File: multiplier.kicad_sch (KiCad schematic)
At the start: 4 parts, among them U12 4081, U2 4081, U37 4069, U7 4081

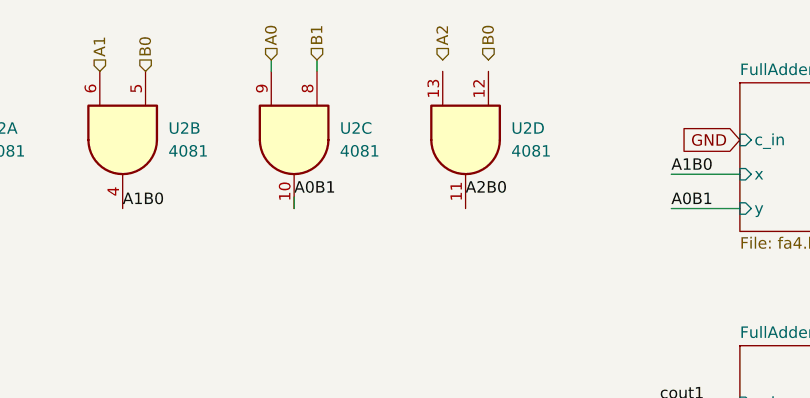
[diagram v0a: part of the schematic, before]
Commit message: Add files via upload
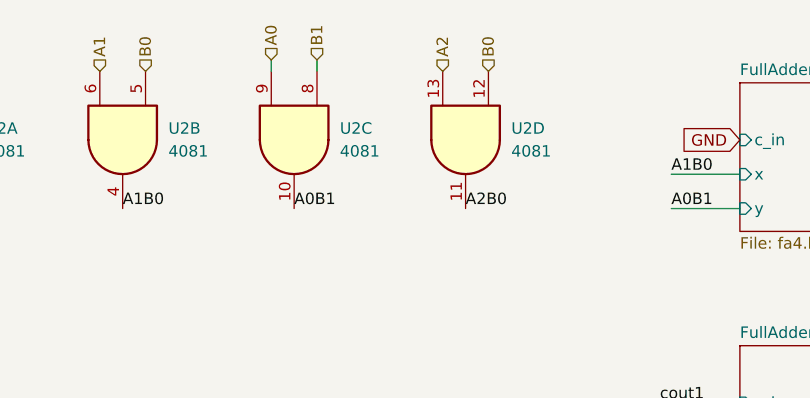
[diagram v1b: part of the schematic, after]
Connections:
- net A2: now also U2.13
- net A2B0: now also U2.11
- net B0: now also U2.12
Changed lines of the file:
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@@
-	(wire
-		(pts
-			(xy 71.12 48.26) (xy 71.12 46.99)
-		)
-		(stroke
-			(width 0)
-			(type default)
-		)
-	)
 	(wire
 		(pts
@@
 	)
 	(label "A2B0"
-		(at 90.17 46.99 0)
+		(at 90.17 48.26 0)
 		(effects
 			(font
@@
 	)
 	(label "A0B1"
-		(at 71.12 46.99 0)
+		(at 71.12 48.26 0)
 		(effects
 			(font
@@
 	(hierarchical_label "B0"
 		(shape input)
-		(at 92.71 31.75 90)
+		(at 92.71 33.02 90)
 		(effects
 			(font
@@
 	(hierarchical_label "A2"
 		(shape input)
-		(at 87.63 31.75 90)
-		(effects
-			(font
+		(at 87.63 33.02 90)
+		(effects
+			(font
